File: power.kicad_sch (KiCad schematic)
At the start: 14 parts, among them J3 Conn_01x02, U1 TP4056-42-ESOP8, U11 TPS62170DSG

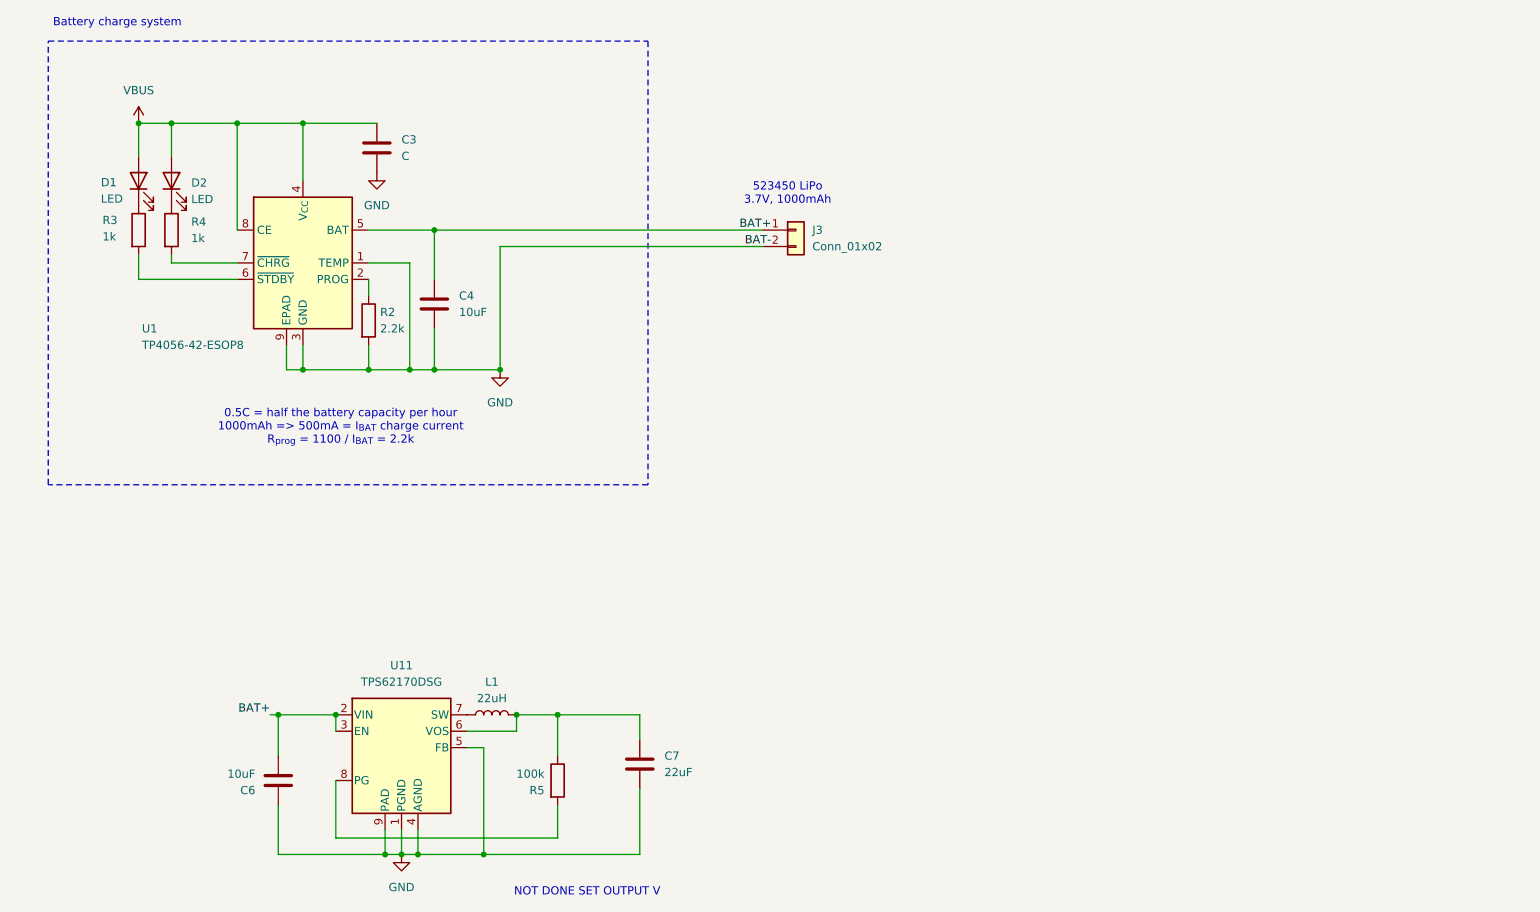
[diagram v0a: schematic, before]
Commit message: finish power management
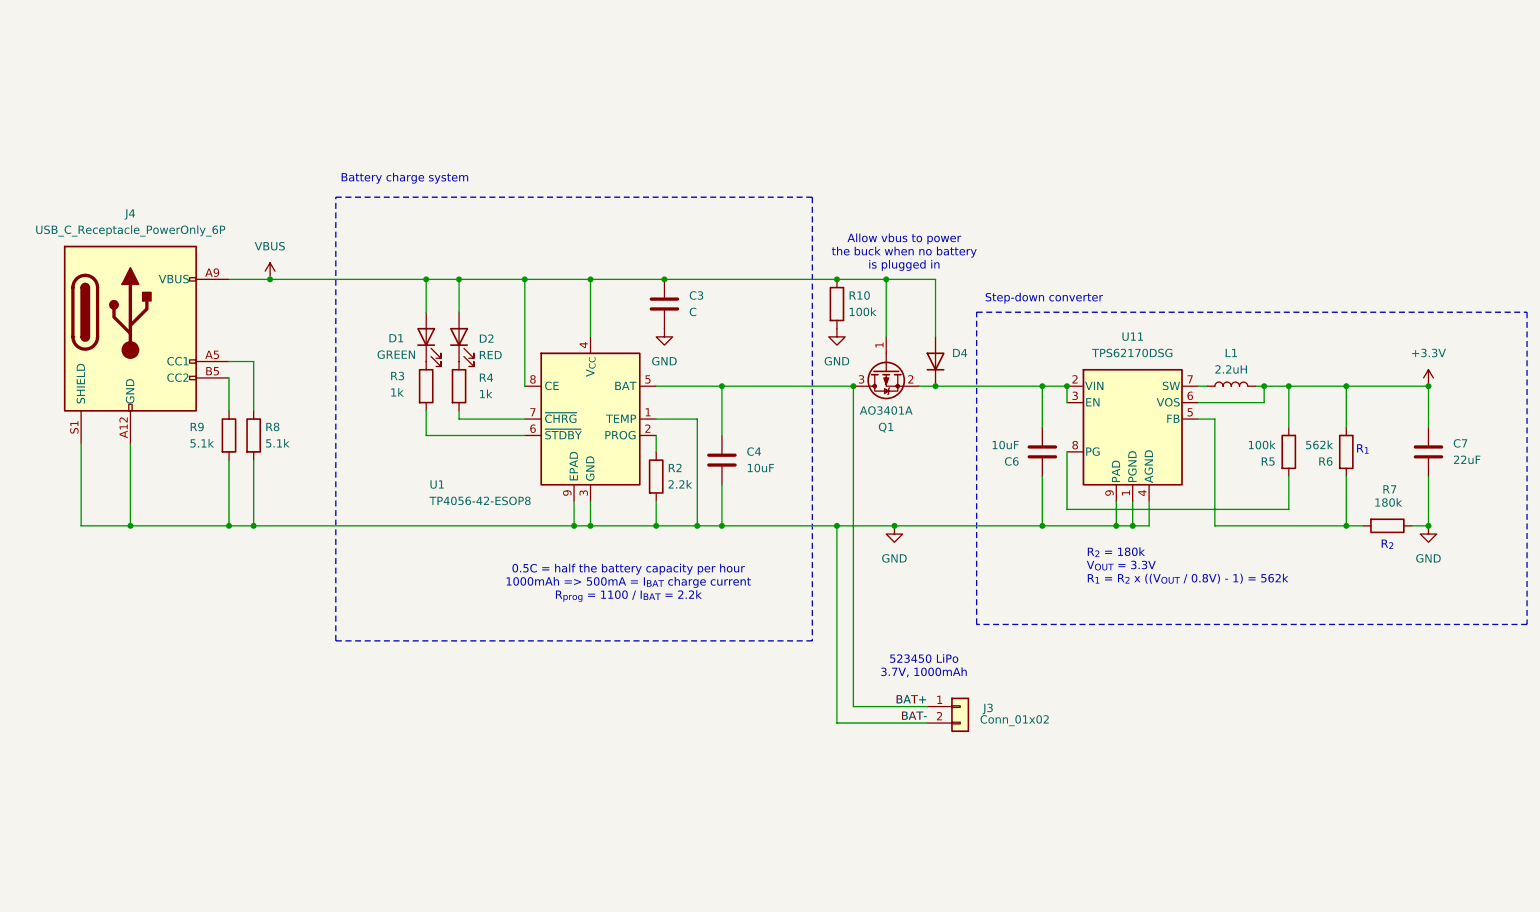
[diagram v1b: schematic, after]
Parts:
- added D4: D, symbol Device:D
- added J4: USB_C_Receptacle_PowerOnly_6P, symbol Connector:USB_C_Receptacle_PowerOnly_6P
- added Q1: AO3401A, Package_TO_SOT_SMD:SOT-23, symbol Transistor_FET:AO3401A
- added R10: 100k, Resistor_SMD:R_0603_1608Metric, symbol Device:R
- added R6: 562k, Resistor_SMD:R_0603_1608Metric, symbol Device:R
- added R7: 180k, Resistor_SMD:R_0603_1608Metric, symbol Device:R
- added R8, R9: 5.1k, Resistor_SMD:R_0603_1608Metric, symbol Device:R
- C3, C4, C6, C7: footprint (none) -> Capacitor_SMD:C_0603_1608Metric
- D1: value LED -> GREEN; footprint (none) -> LED_SMD:LED_0603_1608Metric; LCSC (none) -> C965804; Manufacturer (none) -> XINGLIGHT; Manufacturer Part Number (none) -> XL-1608UGC-04
- D2: value LED -> RED; footprint (none) -> LED_SMD:LED_0603_1608Metric; LCSC (none) -> C965799; Manufacturer (none) -> XINGLIGHT; Manufacturer Part Number (none) -> XL-1608SURC-06
- J3: LCSC (none) -> C131337; Manufacturer (none) -> JST; Manufacturer Part Number (none) -> B2B-PH-K-S(LF)(SN)
- L1: value 22uH -> 2.2uH; LCSC C128694 -> C5349701; Manufacturer SXN -> APV; Manufacturer Part Number SMMS0630-220M -> APH0630T2R2M
- R2, R3, R4, R5: footprint (none) -> Resistor_SMD:R_0603_1608Metric
- U1: LCSC (none) -> C16581; Manufacturer (none) -> TOP POWER ASIC; Manufacturer Part Number (none) -> TP4056-42-ESOP8
- U11: LCSC (none) -> TI; Manufacturer (none) -> C124041; Manufacturer Part Number (none) -> TPS62170DSGR
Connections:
- net BAT+: now also C4.1, J3.1 (Pin_1), U1.5 (BAT), Q1.3 (D); no longer C6.1, U11.2 (VIN), U11.3 (EN)
- net GND: now also J4.A12 (GND), J4.B12 (GND), J4.S1 (SHIELD), R10.2, R7.1, R8.2, R9.2; no longer U11.5 (FB)
- net VBUS: now also D4.2 (A), J4.A9 (VBUS), J4.B9 (VBUS), Q1.1 (G), R10.1
- net +3.3V: now reaches C7.1, L1.2, R5.1, U11.6 (VOS)
- net +3.3V: now also R6.1
- new net: C6.1, D4.1 (K), Q1.2 (S), U11.2 (VIN), U11.3 (EN)
- new net: R6.2, R7.2, U11.5 (FB)
- new net: J4.A5 (CC1), R8.1
- new net: J4.B5 (CC2), R9.1
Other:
- note added: "Allow vbus to power the buck when no battery is plugged in"
- note added: "R_{1}"
- note added: "R_{2}"
- note added: "R_{2} = 180k V_{OUT} = 3.3V R_{1} = R_{2} x ((V_{OUT} / 0.8V) - 1) = 562k"
- note added: "Step-down converter"
- note removed: "NOT DONE SET OUTPUT V"
- moved on the sheet: C3, C4, C6, C7, D1, D2, J3, L1, R2, R3, R4, R5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

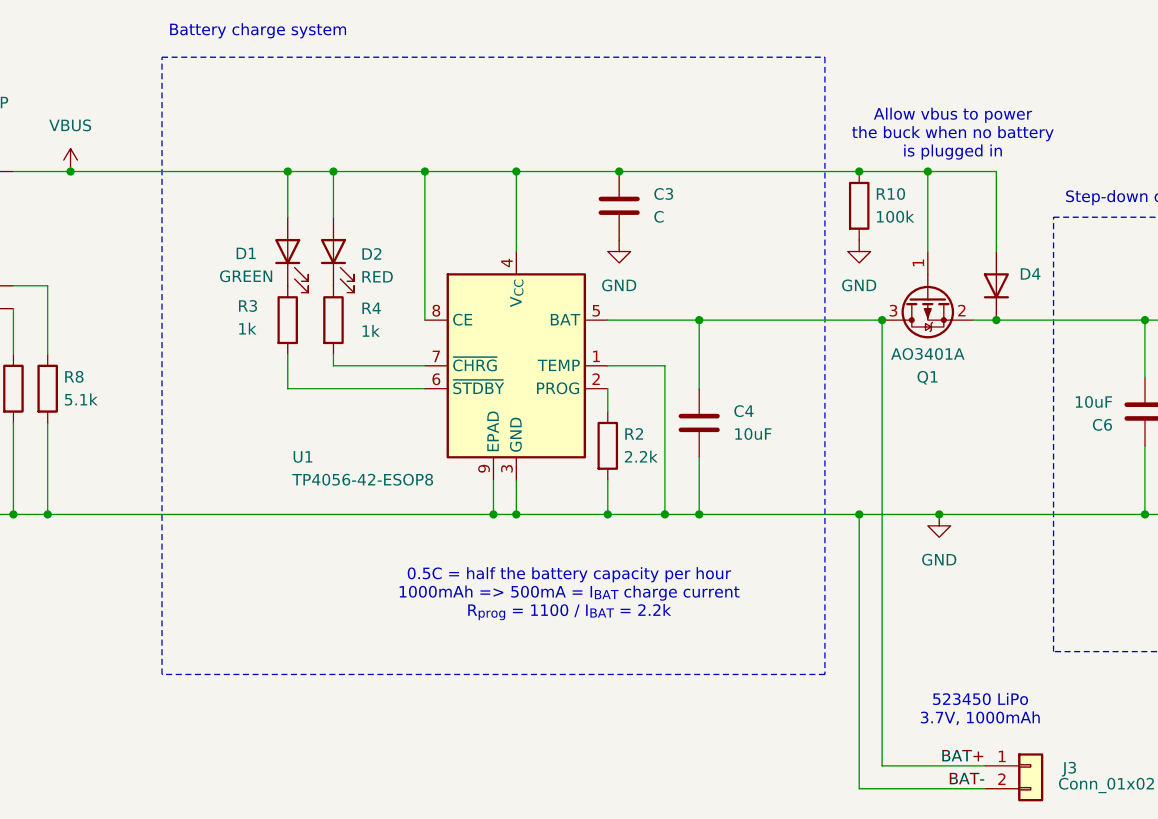
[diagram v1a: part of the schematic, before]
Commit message: led driver backlight, not finished
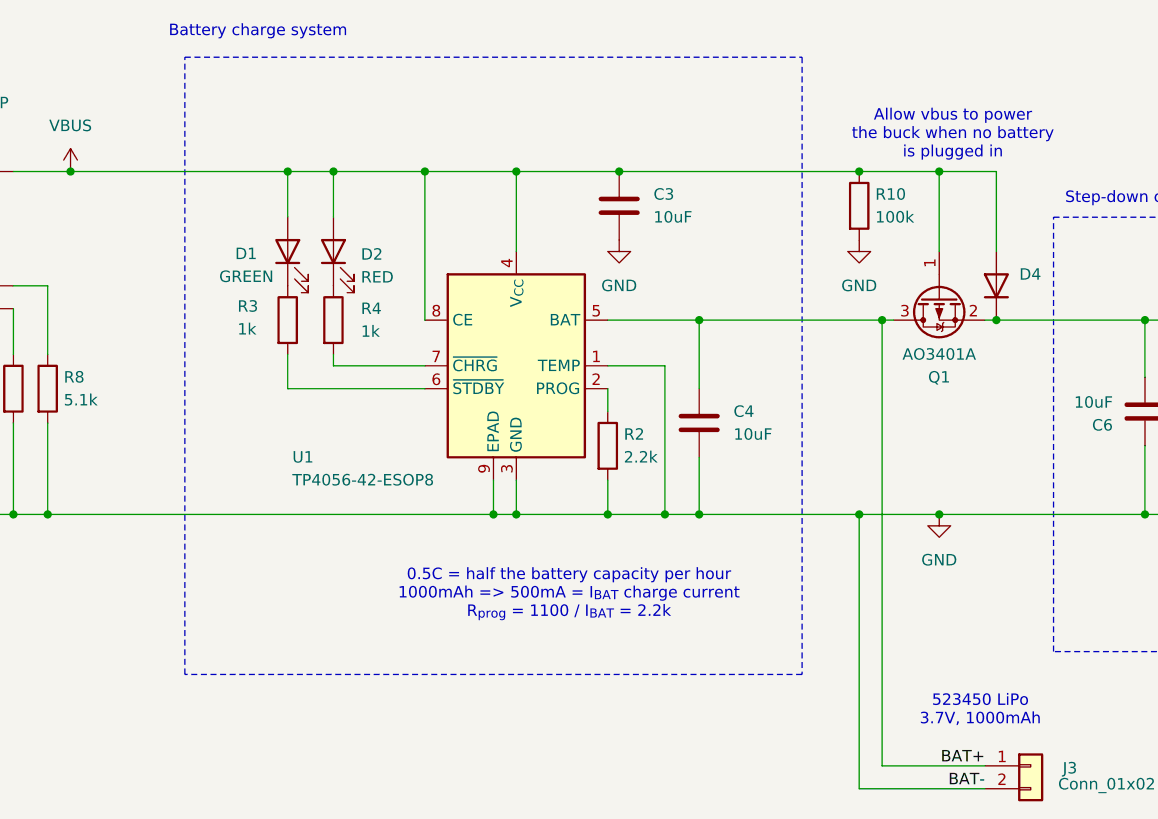
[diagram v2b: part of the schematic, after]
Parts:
- C3: value C -> 10uF
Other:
- moved on the sheet: Q1
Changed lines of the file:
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@@
 	)
 	(rectangle
-		(start 78.74 53.34)
-		(end 152.4 121.92)
+		(start 81.28 53.34)
+		(end 149.86 121.92)
 		(stroke
 			(width 0)
@@
 	)
 	(junction
-		(at 163.83 66.04)
-		(diameter 0)
-		(color 0 0 0 0)
-	)
-	(junction
 		(at 201.93 104.14)
 		(diameter 0)
@@
 	)
 	(junction
+		(at 165.1 66.04)
+		(diameter 0)
+		(color 0 0 0 0)
+	)
+	(junction
 		(at 68.58 66.04)
 		(diameter 0)
@@
 	(wire
 		(pts
-			(xy 163.83 66.04) (xy 171.45 66.04)
+			(xy 214.63 87.63) (xy 214.63 104.14)
 		)
 		(stroke
@@
 	(wire
 		(pts
-			(xy 214.63 87.63) (xy 214.63 104.14)
+			(xy 165.1 66.04) (xy 171.45 66.04)
 		)
 		(stroke
@@
 	(wire
 		(pts
-			(xy 163.83 66.04) (xy 163.83 74.93)
+			(xy 165.1 66.04) (xy 165.1 74.93)
 		)
 		(stroke
@@
 	(wire
 		(pts
+			(xy 160.02 82.55) (xy 158.75 82.55)
+		)
+		(stroke
+			(width 0)
+			(type default)
+		)
+	)
+	(wire
+		(pts
 			(xy 212.09 85.09) (xy 222.25 85.09)
 		)
@@
 	(wire
 		(pts
-			(xy 168.91 82.55) (xy 171.45 82.55)
+			(xy 170.18 82.55) (xy 171.45 82.55)
 		)
 		(stroke
@@
 	(wire
 		(pts
-			(xy 156.21 66.04) (xy 163.83 66.04)
+			(xy 156.21 66.04) (xy 165.1 66.04)
 		)
 		(stroke
@@
 			)
 		)
-		(property "Value" "C"
+		(property "Value" "10uF"
 			(at 133.35 71.1199 0)
 			(effects
@@
 	(symbol
 		(lib_id "Transistor_FET:AO3401A")
-		(at 163.83 80.01 90)
+		(at 165.1 80.01 90)
 		(mirror x)
 		(unit 1)
@@
 		(dnp no)
 		(property "Reference" "Q1"
-			(at 163.83 88.9 90)
+			(at 165.1 88.9 90)
 			(effects
 				(font
@@
 		)
 		(property "Value" "AO3401A"
-			(at 163.83 86.36 90)
+			(at 165.1 86.36 90)
 			(effects
 				(font
@@
 		)
 		(property "Footprint" "Package_TO_SOT_SMD:SOT-23"
-			(at 165.735 85.09 0)
+			(at 167.005 85.09 0)
 			(effects
 				(font
@@
 		)
 		(property "Datasheet" "http://www.aosmd.com/pdfs/datasheet/AO3401A.pdf"
-			(at 167.64 85.09 0)
+			(at 168.91 85.09 0)
 			(effects
 				(font
@@
 		)
 		(property "Description" "-4.0A Id, -30V Vds, P-Channel MOSFET, SOT-23"
-			(at 163.83 80.01 0)
+			(at 165.1 80.01 0)
 			(effects
 				(font
@@
 		)
 		(property "LCSC" "C347476"
-			(at 163.83 80.01 0)
+			(at 165.1 80.01 0)
 			(effects
 				(font
@@
 		)
 		(property "Manufacturer" "UMW"
-			(at 163.83 80.01 0)
+			(at 165.1 80.01 0)
 			(effects
 				(font
@@
 		)
 		(property "Manufacturer Part Number" "AO3401A"
-			(at 163.83 80.01 0)
+			(at 165.1 80.01 0)
 			(effects
 				(font
